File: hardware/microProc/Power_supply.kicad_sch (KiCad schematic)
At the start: 5 parts, among them U2 BU33SD5WG-TR

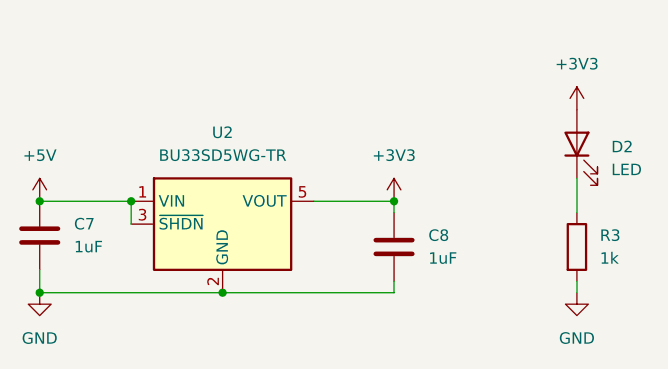
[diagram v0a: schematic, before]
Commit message: Routage carte
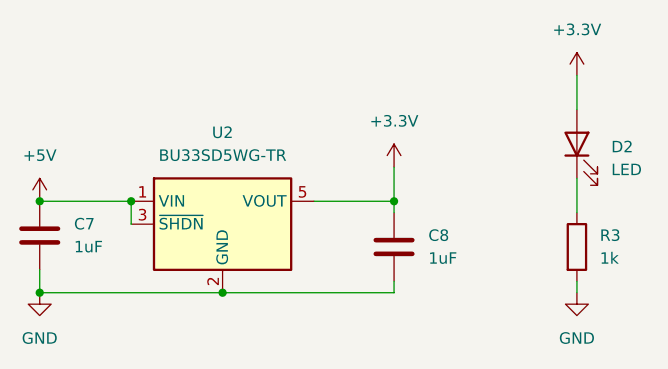
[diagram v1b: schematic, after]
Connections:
- net +3V3 renamed +3.3V
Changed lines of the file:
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@@
   (junction (at 125.73 77.47) (diameter 0) (color 0 0 0 0)
   )
+  (junction (at 165.1 77.47) (diameter 0) (color 0 0 0 0)
+  )
   (junction (at 146.05 87.63) (diameter 0) (color 0 0 0 0)
-  )
-  (junction (at 165.1 77.47) (diameter 0) (color 0 0 0 0)
   )
   (wire (pts (xy 185.42 74.93) (xy 185.42 78.74))
@@
     (stroke (width 0) (type default) (color 0 0 0 0))
   )
+  (wire (pts (xy 165.1 73.66) (xy 165.1 77.47))
+    (stroke (width 0) (type default) (color 0 0 0 0))
+  )
   (wire (pts (xy 185.42 86.36) (xy 185.42 87.63))
     (stroke (width 0) (type default) (color 0 0 0 0))
@@
   )
   (wire (pts (xy 135.89 80.01) (xy 135.89 77.47))
+    (stroke (width 0) (type default) (color 0 0 0 0))
+  )
+  (wire (pts (xy 185.42 63.5) (xy 185.42 67.31))
     (stroke (width 0) (type default) (color 0 0 0 0))
   )
@@
     (pin "2")
   )
-  (symbol (lib_id "power:+3V3") (at 185.42 67.31 0) (unit 1)
+  (symbol (lib_id "power:+3.3V") (at 165.1 73.66 0) (unit 1)
     (in_bom yes) (on_board yes) (fields_autoplaced)
-    (property "Reference" "#PWR014" (id 0) (at 185.42 71.12 0)
+    (property "Reference" "#PWR?" (id 0) (at 165.1 77.47 0)
       (effects (font (size 1.27 1.27)) hide)
     )
-    (property "Value" "+3V3" (id 1) (at 185.42 62.23 0))
-    (property "Footprint" "" (id 2) (at 185.42 67.31 0)
+    (property "Value" "+3.3V" (id 1) (at 165.1 68.58 0))
+    (property "Footprint" "" (id 2) (at 165.1 73.66 0)
       (effects (font (size 1.27 1.27)) hide)
     )
-    (property "Datasheet" "" (id 3) (at 185.42 67.31 0)
-      (effects (font (size 1.27 1.27)) hide)
-    )
-    (pin "1")
-  )
-  (symbol (lib_id "power:+3V3") (at 165.1 77.47 0) (unit 1)
-    (in_bom yes) (on_board yes) (fields_autoplaced)
-    (property "Reference" "#PWR013" (id 0) (at 165.1 81.28 0)
-      (effects (font (size 1.27 1.27)) hide)
-    )
-    (property "Value" "+3V3" (id 1) (at 165.1 72.39 0))
-    (property "Footprint" "" (id 2) (at 165.1 77.47 0)
-      (effects (font (size 1.27 1.27)) hide)
-    )
-    (property "Datasheet" "" (id 3) (at 165.1 77.47 0)
+    (property "Datasheet" "" (id 3) (at 165.1 73.66 0)
       (effects (font (size 1.27 1.27)) hide)
     )
@@
     (pin "2")
   )
+  (symbol (lib_id "power:+3.3V") (at 185.42 63.5 0) (unit 1)
+    (in_bom yes) (on_board yes) (fields_autoplaced)
+    (property "Reference" "#PWR?" (id 0) (at 185.42 67.31 0)
+      (effects (font (size 1.27 1.27)) hide)
+    )
+    (property "Value" "+3.3V" (id 1) (at 185.42 58.42 0))
+    (property "Footprint" "" (id 2) (at 185.42 63.5 0)
+      (effects (font (size 1.27 1.27)) hide)
+    )
+    (property "Datasheet" "" (id 3) (at 185.42 63.5 0)
+      (effects (font (size 1.27 1.27)) hide)
+    )
+    (pin "1")
+  )
   (symbol (lib_id "Device:C") (at 125.73 81.28 0) (unit 1)
